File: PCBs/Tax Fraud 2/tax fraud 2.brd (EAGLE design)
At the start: 100 x 80 mm, 7 parts, among them J1 USB4105-GF-A, U1 RFM95W-915S2

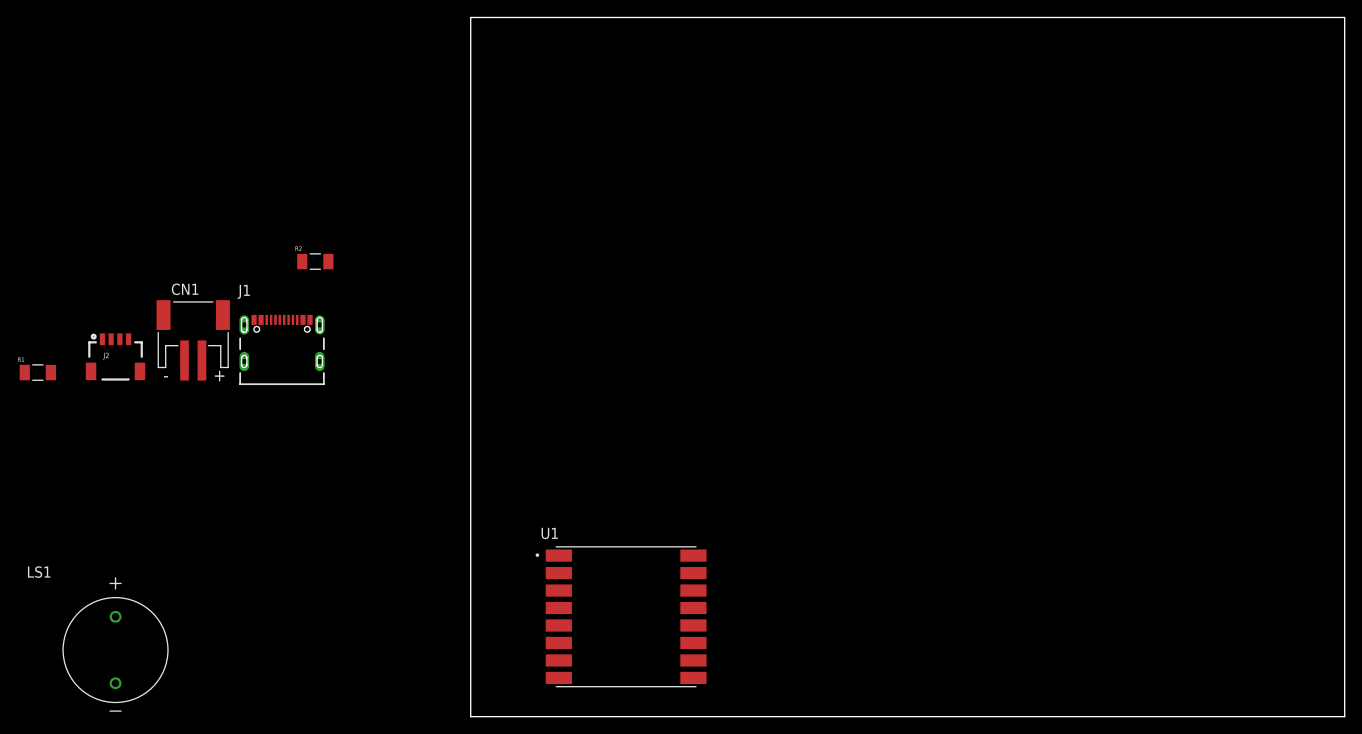
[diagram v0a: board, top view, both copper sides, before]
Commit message: TF2 autosave
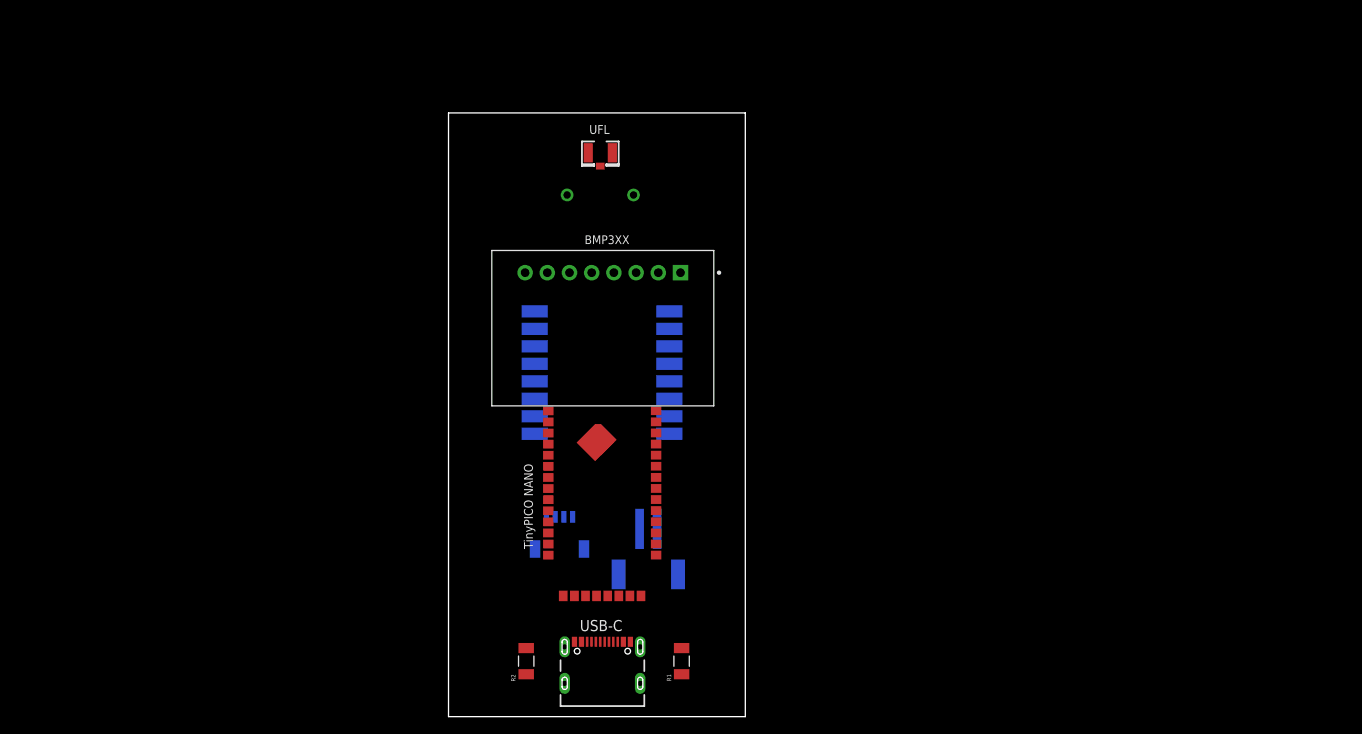
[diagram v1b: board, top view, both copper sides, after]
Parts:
- removed CN1: (no value), adafruit:JST-PH-2-SMT-RA
- removed J1: USB4105-GF-A, USB-C Adafruit USB4105-GF-A:GCT_USB4105-GF-A
- removed J2: (no value), SparkFun-Connectors:1X04_1MM_RA
- removed LS1: AI-1223-TWT-12V-R, buzzer:XDCR_AI-1223-TWT-12V-R
- added BEEPER: AI-1223-TWT-12V-R, buzzer:XDCR_AI-1223-TWT-12V-R
- added BMP3XX: ADAFRUIT_INDUSTRIES_3966ADAFRUIT_INDUSTRIES_3966_0_0, BMP388 Breakout:ADAFRUIT_INDUSTRIES_3966_0
- added JST-PH: (no value), adafruit:JST-PH-2-SMT-RA
- added QWIIC: (no value), SparkFun-Connectors:1X04_1MM_RA
- added U$1: TINYPICO-NANO-CONNECTOR, TinyPICO_NANO_Eagle:TINYPICO-NANO-CONNECTOR
- added UFL: (no value), adafruit:U.FL
- added USB-C: USB4105-GF-A, USB-C Adafruit USB4105-GF-A:GCT_USB4105-GF-A
- moved R1 80.7 mm to (24.1, 6.35), turned to 270 degrees
- moved R2 51.7 mm to (6.35, 6.35), turned to 90 degrees
- moved U1 28.1 mm to (15.0, 39.4), flipped to the bottom
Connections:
- removed net 3.3V: U1.13
- removed net N$3: CN1.1, CN1.2, J1.A1_B12, J1.B1_A12, U1.1, U1.10, U1.8
- removed net VBUS: J1.A4_B9, J1.B4_A9
- new net 3VO: BMP3XX.2
- new net ANT: U1.9, UFL.3
- new net CS: U$1.IO5, U1.5
- new net DN: U$1.D-, USB-C.A7, USB-C.B7
- new net DP: U$1.D+, USB-C.A6, USB-C.B6
- new net GPIO9: BEEPER.P, U$1.IO9
- new net MISO: U$1.IO19, U1.2
- new net MOSI: U$1.IO23, U1.3
- new net N$4: U$1.IO36
- new net RST: U$1.IO0, U1.6
- new net SCK: U$1.IO18, U1.4
- new net SCL: BMP3XX.4, QWIIC.4, U$1.IO22
- new net SDA: BMP3XX.6, QWIIC.3, U$1.IO21
- new net VBAT: JST-PH.1, U$1.VBAT
- new net VIN: U$1.5V, USB-C.A4_B9, USB-C.B4_A9
- net GND: now also BEEPER.N, BMP3XX.3, JST-PH.2, QWIIC.1, R1.2, R2.1, U$1.GND$1, U$1.GND$2, U$1.GND$3, U$1.GND$4, U1.1, U1.10, U1.8, UFL.1, UFL.2, USB-C.A1_B12, USB-C.B1_A12; no longer J2.1
- net N$1: now also R1.1, USB-C.B5; no longer J1.A5, R1.2
- net N$2: now also USB-C.A5; no longer J1.B5
- net SHELL_GND: now also USB-C.S1, USB-C.S2, USB-C.S3, USB-C.S4; no longer J1.S1, J1.S2, J1.S3, J1.S4
- net VCC: now also BMP3XX.1, QWIIC.2, U$1.3V3, U1.13; no longer J2.2
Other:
- board size 100 x 80 mm -> 34 x 69.1 mm
- board text added: "ANT"
- board text added: "GND"
- board text added: "TinyPICO NANO"
